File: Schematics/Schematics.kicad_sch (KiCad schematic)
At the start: 18 parts, among them J1 BAT, U1 TP4056, U2 BH1750, U3 BME688, U4 BU30TD3WG, U5 NRF52840-DONGLE, U6 LIS3DH

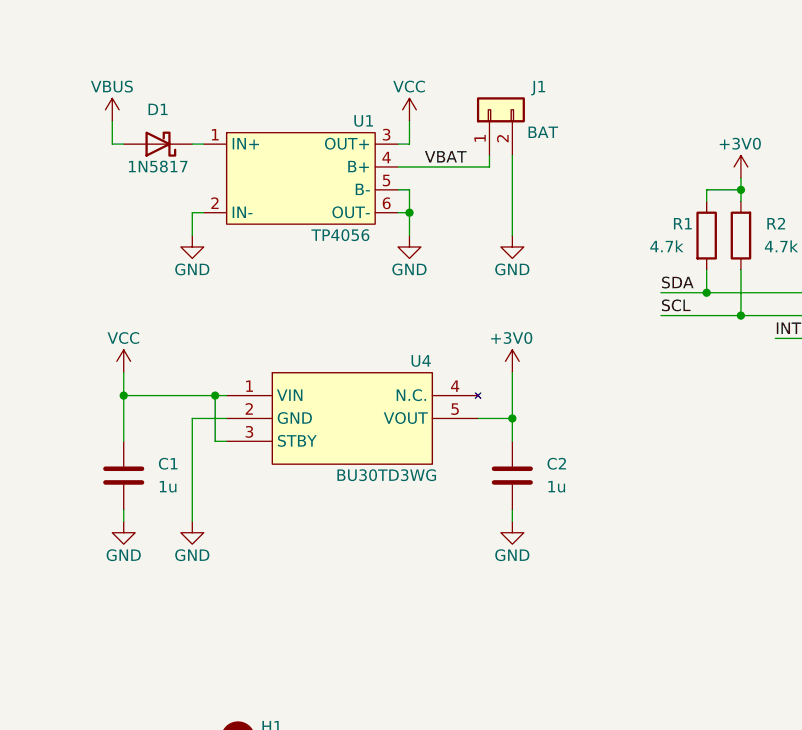
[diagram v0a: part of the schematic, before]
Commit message: Uploading Modified Schematic with PCB version 1
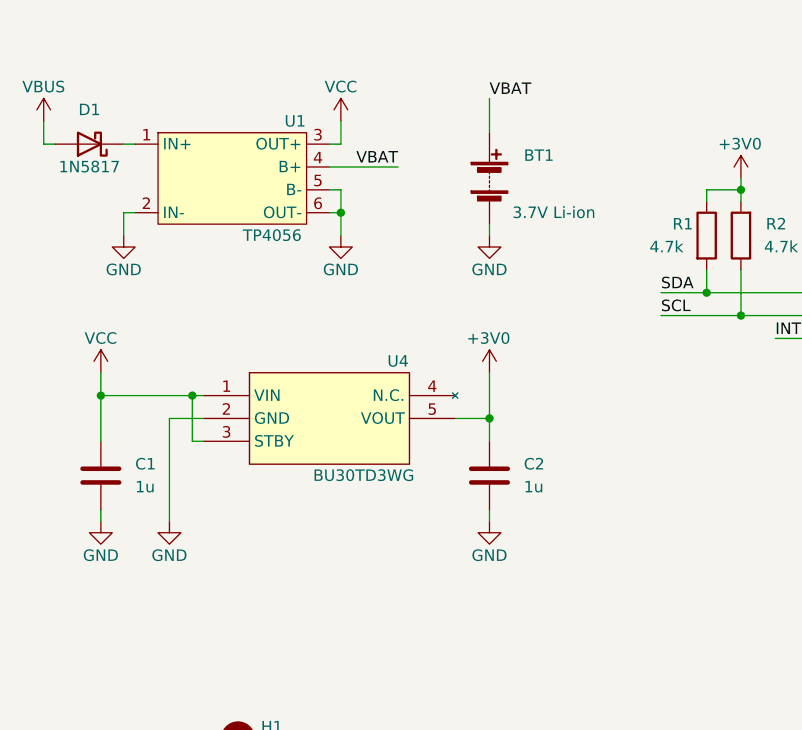
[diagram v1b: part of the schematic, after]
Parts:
- removed J1: BAT, custom:KLS5-18650-005, symbol Connector_Generic:Conn_01x02
- added BT1: 3.7V Li-ion, custom:KLS5-18650-005, symbol Device:Battery
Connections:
- net GND: now also BT1.2 (-)
- net VBAT: now also BT1.1 (+)
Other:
- moved on the sheet: C1, C2, D1, U1, U4
